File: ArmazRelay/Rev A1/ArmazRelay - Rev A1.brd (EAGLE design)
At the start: 70 x 30 mm, 9 parts, among them J1 MSTBA2, J2 MSTBA3, J3 22-05-7038-03, J4 22-05-7038-03, K1 MY2, T1 EXMACHINA-LOGO-NAME

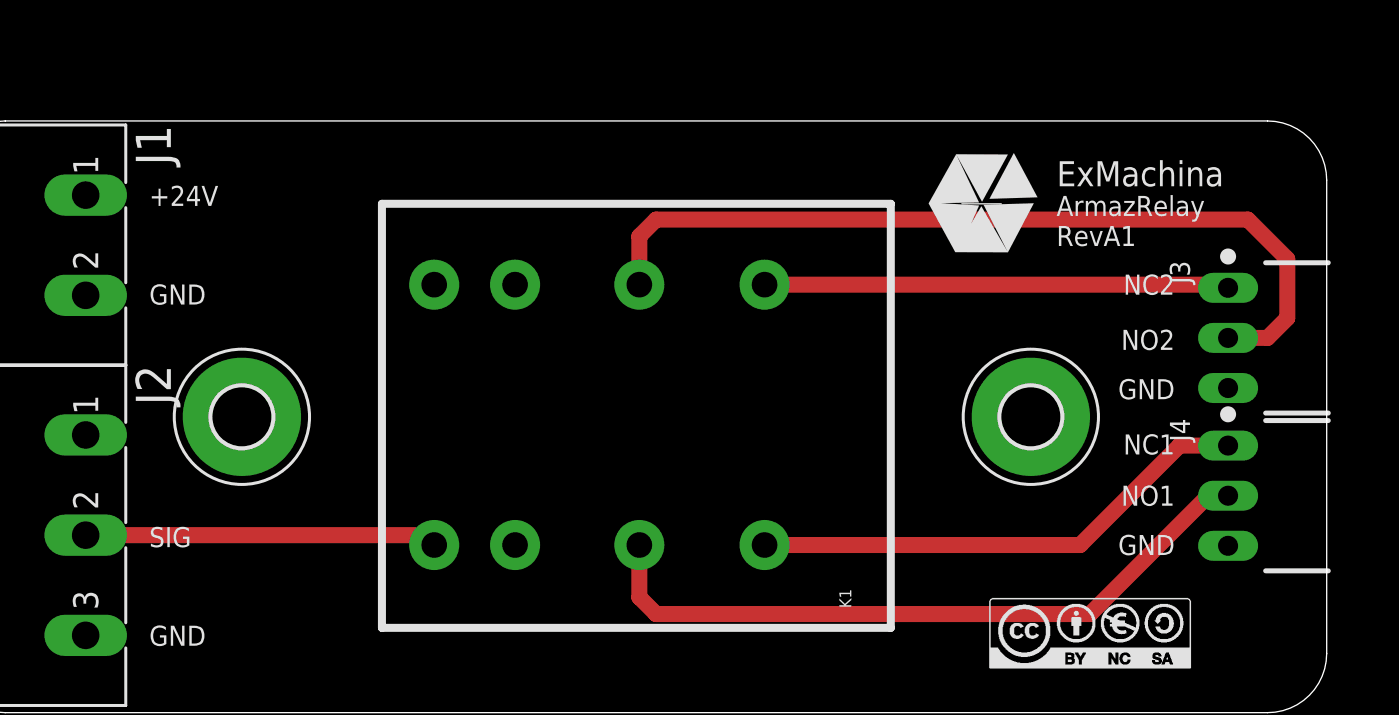
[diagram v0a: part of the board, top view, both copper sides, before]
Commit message: Generate MDP files
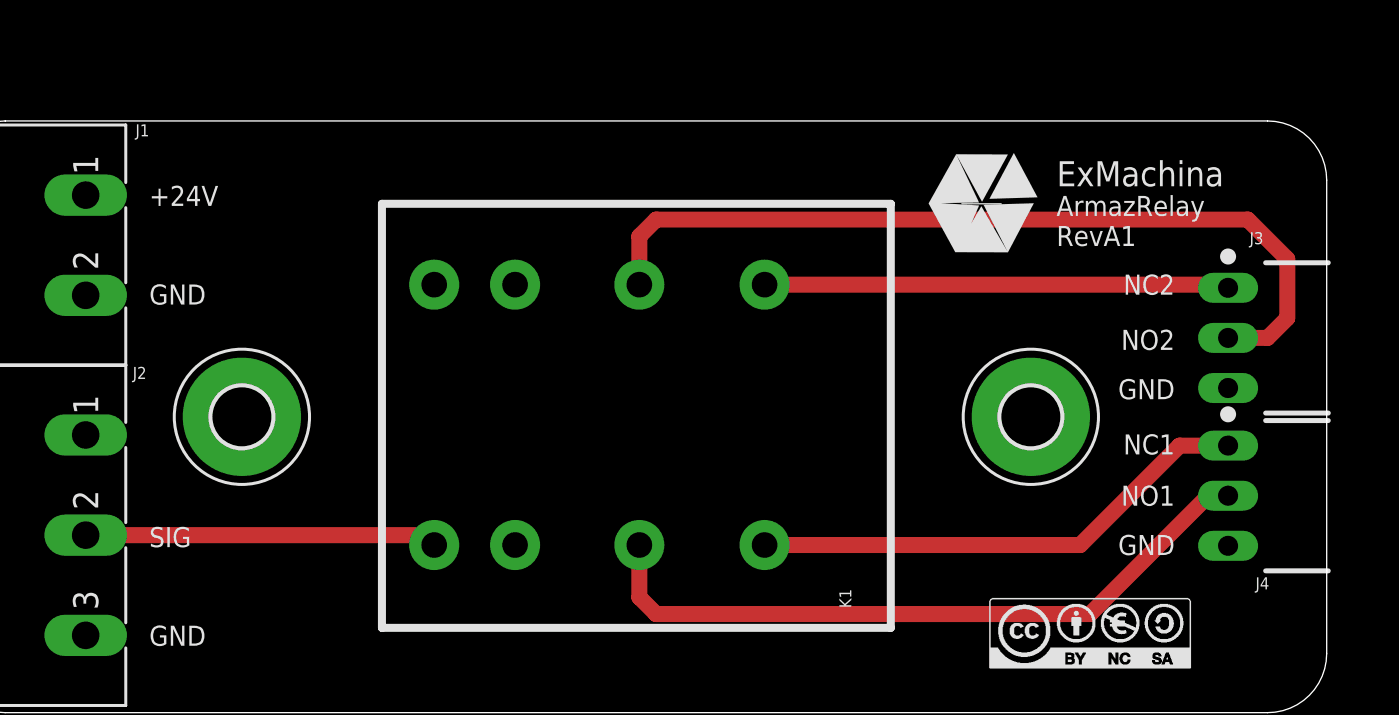
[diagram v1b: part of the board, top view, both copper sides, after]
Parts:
- added U$1: (no value), frames:A4L-LOC
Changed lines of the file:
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@@
 <setting verticaltext="up"/>
 </settings>
-<grid distance="1" unitdist="mm" unit="mm" style="lines" multiple="1" display="no" altdistance="0.1" altunitdist="mm" altunit="mm"/>
+<grid distance="1" unitdist="mm" unit="mil" style="lines" multiple="1" display="no" altdistance="0.1" altunitdist="mm" altunit="mm"/>
 <layers>
-<layer number="1" name="Top" color="4" fill="1" visible="yes" active="yes"/>
+<layer number="1" name="Top" color="4" fill="1" visible="no" active="yes"/>
 <layer number="2" name="Route2" color="1" fill="3" visible="no" active="no"/>
 <layer number="3" name="Route3" color="4" fill="3" visible="no" active="no"/>
 <layer number="14" name="Route14" color="1" fill="6" visible="no" active="no"/>
 <layer number="15" name="Route15" color="4" fill="6" visible="no" active="no"/>
-<layer number="16" name="Bottom" color="1" fill="1" visible="yes" active="yes"/>
-<layer number="17" name="Pads" color="2" fill="1" visible="yes" active="yes"/>
-<layer number="18" name="Vias" color="2" fill="1" visible="yes" active="yes"/>
+<layer number="16" name="Bottom" color="1" fill="1" visible="no" active="yes"/>
+<layer number="17" name="Pads" color="2" fill="1" visible="no" active="yes"/>
+<layer number="18" name="Vias" color="2" fill="1" visible="no" active="yes"/>
 <layer number="19" name="Unrouted" color="6" fill="1" visible="yes" active="yes"/>
 <layer number="20" name="Dimension" color="15" fill="1" visible="yes" active="yes"/>
 <layer number="21" name="tPlace" color="7" fill="1" visible="yes" active="yes"/>
-<layer number="22" name="bPlace" color="7" fill="1" visible="yes" active="yes"/>
+<layer number="22" name="bPlace" color="7" fill="1" visible="no" active="yes"/>
 <layer number="23" name="tOrigins" color="15" fill="1" visible="yes" active="yes"/>
-<layer number="24" name="bOrigins" color="15" fill="1" visible="yes" active="yes"/>
-<layer number="25" name="tNames" color="7" fill="1" visible="no" active="yes"/>
+<layer number="24" name="bOrigins" color="15" fill="1" visible="no" active="yes"/>
+<layer number="25" name="tNames" color="7" fill="1" visible="yes" active="yes"/>
 <layer number="26" name="bNames" color="7" fill="1" visible="no" active="yes"/>
-<layer number="27" name="tValues" color="7" fill="1" visible="no" active="yes"/>
+<layer number="27" name="tValues" color="7" fill="1" visible="yes" active="yes"/>
 <layer number="28" name="bValues" color="7" fill="1" visible="no" active="yes"/>
 <layer number="29" name="tStop" color="7" fill="3" visible="no" active="yes"/>
@@
 <layer number="49" name="Reference" color="7" fill="1" visible="no" active="yes"/>
 <layer number="50" name="dxf" color="7" fill="1" visible="no" active="yes"/>
-<layer number="51" name="tDocu" color="7" fill="1" visible="no" active="yes"/>
+<layer number="51" name="tDocu" color="7" fill="1" visible="yes" active="yes"/>
 <layer number="52" name="bDocu" color="7" fill="1" visible="no" active="yes"/>
 <layer number="53" name="tGND_GNDA" color="7" fill="1" visible="no" active="yes"/>
@@
 <layer number="98" name="Guide" color="6" fill="1" visible="no" active="no"/>
 <layer number="99" name="SpiceOrder" color="7" fill="1" visible="no" active="no"/>
-<layer number="100" name="Mechanical" color="7" fill="1" visible="no" active="yes"/>
+<layer number="100" name="Mechanical" color="7" fill="1" visible="yes" active="yes"/>
 <layer number="101" name="Patch_Top" color="7" fill="1" visible="no" active="yes"/>
 <layer number="102" name="Vscore" color="7" fill="1" visible="no" active="yes"/>
@@
 <wire x1="67" y1="30" x2="3" y2="30" width="0" layer="20"/>
 <wire x1="3" y1="30" x2="0" y2="27" width="0" layer="20" curve="90"/>
-<dimension x1="15" y1="15" x2="55" y2="15" x3="35" y3="-7" textsize="2.54" layer="48"/>
-<dimension x1="35" y1="15" x2="0" y2="15" x3="17.5" y3="34" textsize="2.54" layer="48"/>
-<dimension x1="55.5" y1="15" x2="55.5" y2="30" x3="87" y3="22.5" textsize="2.54" layer="48"/>
-<dimension x1="67" y1="30" x2="58" y2="0" x3="95" y3="15" textsize="2.54" layer="48" dtype="vertical"/>
-<dimension x1="0" y1="3" x2="70" y2="4" x3="35" y3="-14" textsize="2.54" layer="48" dtype="horizontal"/>
 <text x="56.3" y="26.2" size="1.016" layer="21" align="top-left">ArmazRelay
 RevA1</text>
@@
 <text x="62.3" y="11" size="1.016" layer="21" rot="R180" align="center-left">NO1</text>
 <text x="62.3" y="8.5" size="1.016" layer="21" rot="R180" align="center-left">GND</text>
+<dimension x1="0" y1="3" x2="70" y2="5" x3="35" y3="-8" textsize="1.778" layer="47" dtype="horizontal"/>
+<dimension x1="0" y1="27" x2="15" y2="15" x3="7.5" y3="36" textsize="1.778" layer="47" dtype="horizontal"/>
+<dimension x1="15" y1="15" x2="55" y2="15" x3="35" y3="36" textsize="1.778" layer="47" dtype="horizontal"/>
+<dimension x1="3" y1="0" x2="6" y2="30" x3="-14" y3="15" textsize="1.778" layer="47" dtype="vertical"/>
+<dimension x1="15" y1="15" x2="15" y2="0" x3="-9" y3="7.5" textsize="1.778" layer="47" dtype="vertical"/>
 </plain>
 <attributes>
@@
 <element name="H1" library="holes" package="P3,0" value="MOUNT-PAD3,0" x="15" y="15"/>
 <element name="H2" library="holes" package="P3,0" value="MOUNT-PAD3,0" x="55" y="15"/>
-<element name="J2" library="con-phoenix-508" package="MSTBA3" value="MSTBA3" x="2" y="9" rot="R270">
+<element name="J2" library="con-phoenix-508" package="MSTBA3" value="MSTBA3" x="2" y="9" smashed="yes" rot="R270">
 <attribute name="OC_FARNELL" value="3705183" x="2" y="9" size="1.778" layer="27" rot="R270" display="off"/>
 <attribute name="MPN" value="1757255" x="2" y="9" size="1.778" layer="27" rot="R270" display="off"/>
 <attribute name="MF" value="FARNELL" x="2" y="9" size="1.778" layer="27" rot="R270" display="off"/>
 <attribute name="OC_NEWARK" value="71C4162" x="2" y="9" size="1.778" layer="27" rot="R270" display="off"/>
+<attribute name="NAME" x="9.464" y="16.92" size="0.6096" layer="25" ratio="10"/>
+<attribute name="VALUE" x="9.48" y="16.3" size="0.4064" layer="27" ratio="10"/>
 </element>
 <element name="K1" library="rel-omron" package="PY08" value="MY2" x="35" y="15" rot="R90"/>
 <element name="CC1" library="cc-by-sa" package="CC-BY-NC-SA" value="CC-BY-NC-SA" x="58" y="4"/>
 <element name="T1" library="exmachina" package="EXM-LOGO-BASELINE" value="EXMACHINA-LOGO-NAME" x="52.5" y="25.8"/>
-<element name="J1" library="con-phoenix-508" package="MSTBA2" value="MSTBA2" x="2" y="23.7" rot="R270">
+<element name="J1" library="con-phoenix-508" package="MSTBA2" value="MSTBA2" x="2" y="23.7" smashed="yes" rot="R270">
 <attribute name="MF" value="FARNELL" x="2" y="23.7" size="1.778" layer="27" rot="R270" display="off"/>
 <attribute name="OC_NEWARK" value="71C4161" x="2" y="23.7" size="1.778" layer="27" rot="R270" display="off"/>
 <attribute name="OC_FARNELL" value="3705171" x="2" y="23.7" size="1.778" layer="27" rot="R270" display="off"/>
 <attribute name="MPN" value="1757242" x="2" y="23.7" size="1.778" layer="27" rot="R270" display="off"/>
+<attribute name="NAME" x="9.604" y="29.22" size="0.6096" layer="25" ratio="10"/>
+<attribute name="VALUE" x="9.62" y="28.6" size="0.4064" layer="27" ratio="10"/>
 </element>
-<element name="J4" library="con-molex" package="7395-03" value="22-05-7038-03" x="65" y="11" rot="R90">
+<element name="J4" library="con-molex" package="7395-03" value="22-05-7038-03" x="65" y="11" smashed="yes" rot="R90">
 <attribute name="MF" value="" x="65" y="11" size="1.778" layer="27" rot="R90" display="off"/>
 <attribute name="OC_NEWARK" value="unknown" x="65" y="11" size="1.778" layer="27" rot="R90" display="off"/>
 <attribute name="OC_FARNELL" value="9731610 " x="65" y="11" size="1.778" layer="27" rot="R90" display="off"/>
 <attribute name="MPN" value="" x="65" y="11" size="1.778" layer="27" rot="R90" display="off"/>
+<attribute name="NAME" x="66.3899" y="6.2521" size="0.6096" layer="25" ratio="10"/>
+<attribute name="VALUE" x="66.4399" y="5.6721" size="0.4064" layer="27" ratio="10"/>
 </element>
-<element name="J3" library="con-molex" package="7395-03" value="22-05-7038-03" x="65" y="19" rot="R90">
+<element name="J3" library="con-molex" package="7395-03" value="22-05-7038-03" x="65" y="19" smashed="yes" rot="R90">
 <attribute name="OC_FARNELL" value="9731610 " x="65" y="19" size="1.778" layer="27" rot="R90" display="off"/>
 <attribute name="MF" value="" x="65" y="19" size="1.778" layer="27" rot="R90" display="off"/>
 <attribute name="OC_NEWARK" value="unknown" x="65" y="19" size="1.778" layer="27" rot="R90" display="off"/>
 <attribute name="MPN" value="" x="65" y="19" size="1.778" layer="27" rot="R90" display="off"/>
+<attribute name="NAME" x="66.0899" y="23.7521" size="0.6096" layer="25" ratio="10"/>
+<attribute name="VALUE" x="66.1399" y="23.1721" size="0.4064" layer="27" ratio="10"/>
 </element>
+<element name="U$1" library="frames" package="A4L-LOC" value="" x="-87" y="-63"/>
 </elements>
 <signals>
